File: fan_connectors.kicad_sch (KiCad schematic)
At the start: 30 parts, among them Q1 CJ3134KW, Q2 AO3401A, Q3 CJ3134KW, Q4 AO3401A

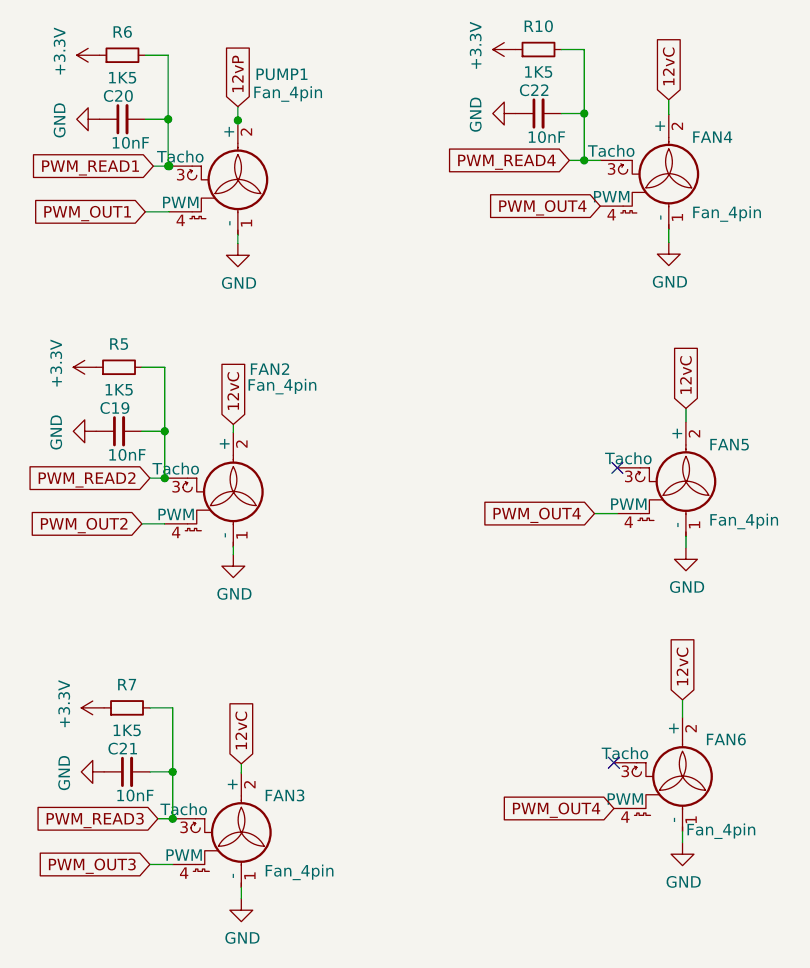
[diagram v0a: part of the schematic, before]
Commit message: kicad - 7
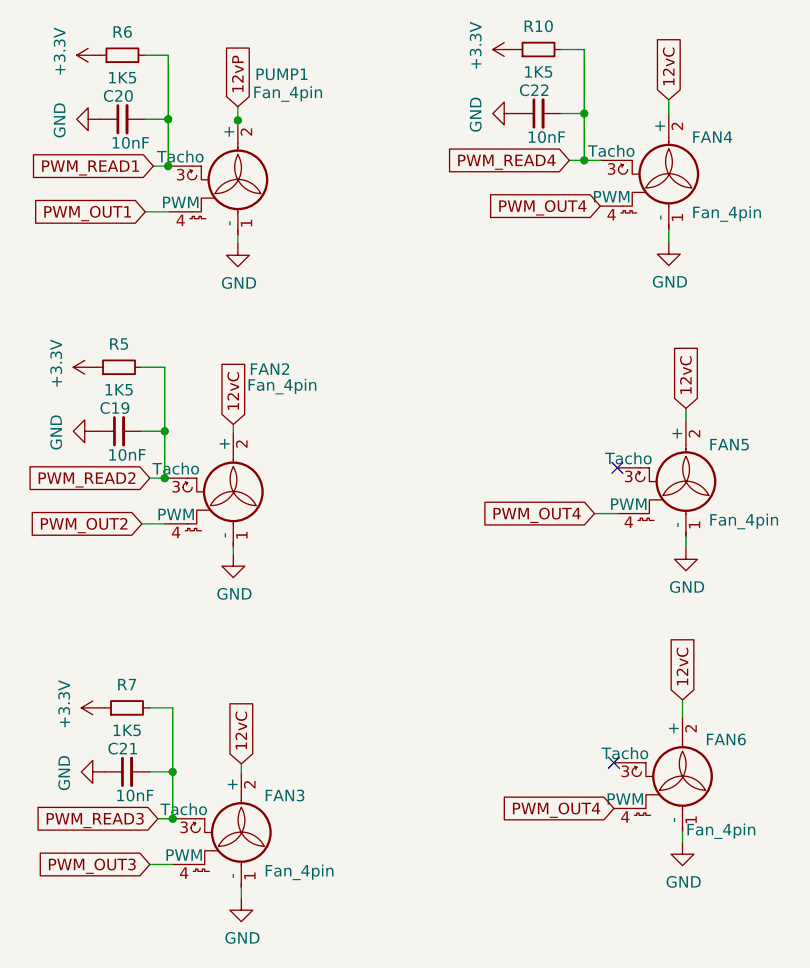
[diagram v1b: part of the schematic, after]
